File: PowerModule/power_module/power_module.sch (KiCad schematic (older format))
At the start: 1 part

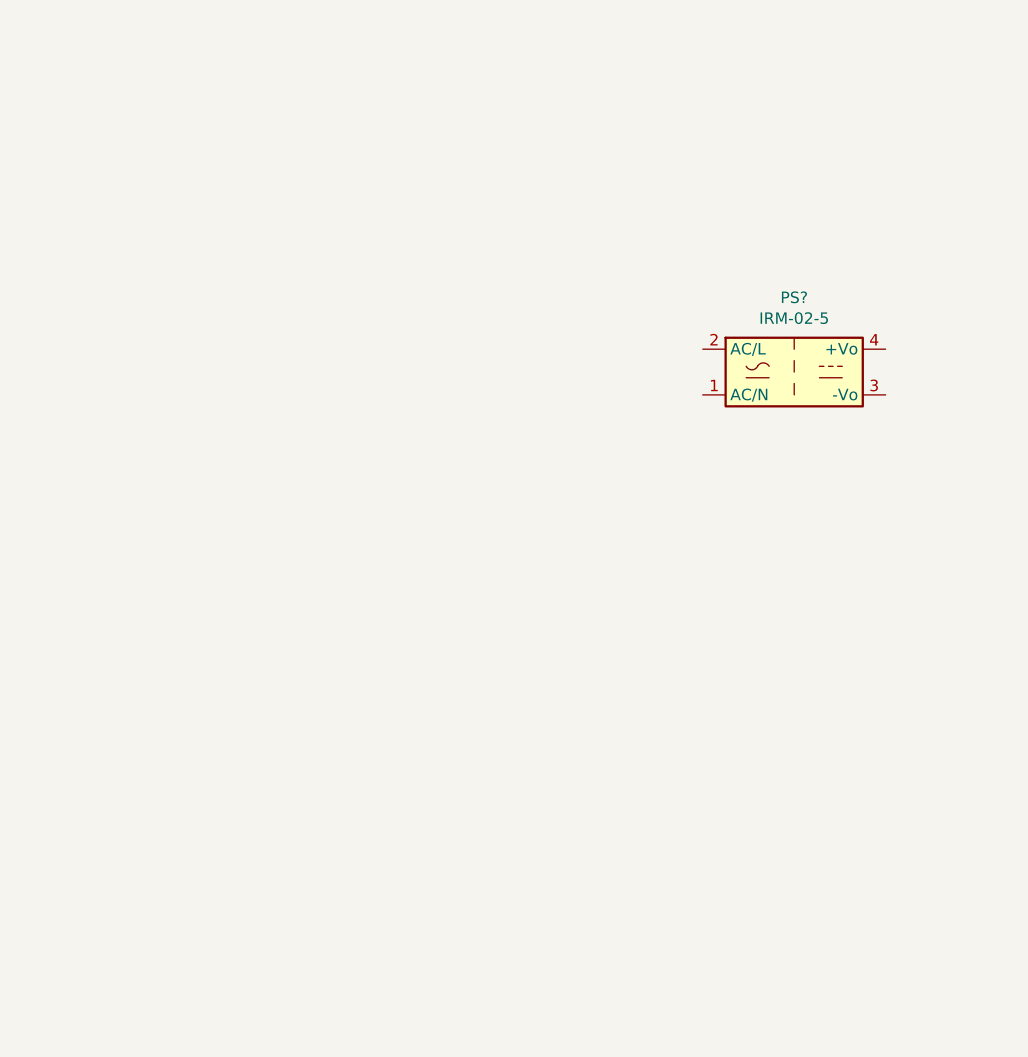
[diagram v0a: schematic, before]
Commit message: Работа над схемой. Добавлены файлы документации на реле
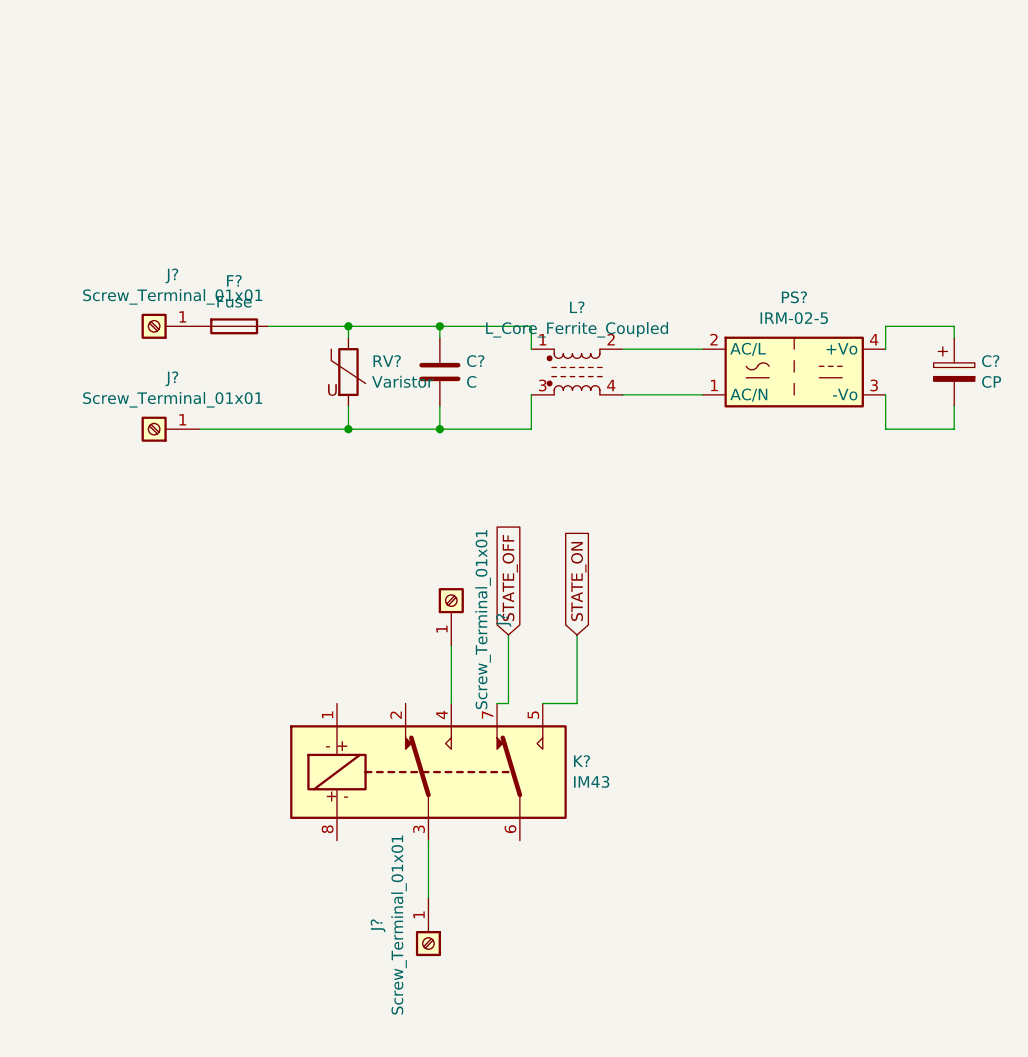
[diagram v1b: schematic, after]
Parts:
- added C?: C, symbol Device:C
- added C?: CP, symbol Device:CP
- added F?: Fuse, symbol Device:Fuse
- added J? (x4): Screw_Terminal_01x01, symbol Connector:Screw_Terminal_01x01
- added K?: IM43, symbol Relay:IM43
- added L?: L_Core_Ferrite_Coupled, symbol Device:L_Core_Ferrite_Coupled
- added RV?: Varistor, symbol Device:Varistor
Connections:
- net at PS?.1 (AC/N): now also L?.4
- net at PS?.2 (AC/L): now also L?.2
- net at PS?.3 (-Vo): now also C?.2
- net at PS?.4 (+Vo): now also C?.1
- new net: C?.1, F?.1, L?.1, RV?.1
- new net: C?.2, J?.1 (Pin_1), L?.3, RV?.2
- new net: F?.2, J?.1 (Pin_1)
- new net: J?.1 (Pin_1), K?.3
- new net: J?.1 (Pin_1), K?.4
- new net STATE_OFF: K?.7
- new net STATE_ON: K?.5
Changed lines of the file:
@@
 	1    0    0    -1
 $EndComp
+$Comp
+L Device:L_Core_Ferrite_Coupled L?
+U 1 1 5FD75833
+P 3000 2750
+F 0 "L?" H 3000 3031 50  0000 C CNN
+F 1 "L_Core_Ferrite_Coupled" H 3000 2940 50  0000 C CNN
+F 2 "" H 3000 2750 50  0001 C CNN
+F 3 "~" H 3000 2750 50  0001 C CNN
+	1    3000 2750
+	1    0    0    -1
+$EndComp
+$Comp
+L Device:C C?
+U 1 1 5FD7B6BD
+P 2400 2750
+F 0 "C?" H 2515 2796 50  0000 L CNN
+F 1 "C" H 2515 2705 50  0000 L CNN
+F 2 "" H 2438 2600 50  0001 C CNN
+F 3 "~" H 2400 2750 50  0001 C CNN
+	1    2400 2750
+	1    0    0    -1
+$EndComp
+$Comp
+L Device:Varistor RV?
+U 1 1 5FD7BDB9
+P 2000 2750
+F 0 "RV?" H 2103 2796 50  0000 L CNN
+F 1 "Varistor" H 2103 2705 50  0000 L CNN
+F 2 "" V 1930 2750 50  0001 C CNN
+F 3 "~" H 2000 2750 50  0001 C CNN
+	1    2000 2750
+	1    0    0    -1
+$EndComp
+$Comp
+L Device:Fuse F?
+U 1 1 5FD7C7CC
+P 1500 2550
+F 0 "F?" V 1303 2550 50  0000 C CNN
+F 1 "Fuse" V 1394 2550 50  0000 C CNN
+F 2 "" V 1430 2550 50  0001 C CNN
+F 3 "~" H 1500 2550 50  0001 C CNN
+	1    1500 2550
+	0    1    1    0
+$EndComp
+Wire Wire Line
+	1650 2550 2000 2550
+Wire Wire Line
+	2400 2550 2400 2600
+Wire Wire Line
+	2000 2600 2000 2550
+Connection ~ 2000 2550
+Wire Wire Line
+	2000 2550 2400 2550
+Wire Wire Line
+	2800 2650 2800 2550
+Wire Wire Line
+	2800 2550 2400 2550
+Connection ~ 2400 2550
+Wire Wire Line
+	2800 2850 2800 3000
+Wire Wire Line
+	2800 3000 2400 3000
+Wire Wire Line
+	2400 3000 2400 2900
+Wire Wire Line
+	2400 3000 2000 3000
+Wire Wire Line
+	2000 3000 2000 2900
+Connection ~ 2400 3000
+$Comp
+L Connector:Screw_Terminal_01x01 J?
+U 1 1 5FD7E4B3
+P 1150 2550
+F 0 "J?" H 1068 2325 50  0000 C CNN
+F 1 "Screw_Terminal_01x01" H 1068 2416 50  0000 C CNN
+F 2 "" H 1150 2550 50  0001 C CNN
+F 3 "~" H 1150 2550 50  0001 C CNN
+	1    1150 2550
+	-1   0    0    1
+$EndComp
+$Comp
+L Connector:Screw_Terminal_01x01 J?
+U 1 1 5FD7F068
+P 1150 3000
+F 0 "J?" H 1068 2775 50  0000 C CNN
+F 1 "Screw_Terminal_01x01" H 1068 2866 50  0000 C CNN
+F 2 "" H 1150 3000 50  0001 C CNN
+F 3 "~" H 1150 3000 50  0001 C CNN
+	1    1150 3000
+	-1   0    0    1
+$EndComp
+Wire Wire Line
+	2000 3000 1350 3000
+Connection ~ 2000 3000
+Wire Wire Line
+	3550 2650 3200 2650
+Wire Wire Line
+	3550 2850 3200 2850
+$Comp
+L Device:CP C?
+U 1 1 5FD807F1
+P 4650 2750
+F 0 "C?" H 4768 2796 50  0000 L CNN
+F 1 "CP" H 4768 2705 50  0000 L CNN
+F 2 "" H 4688 2600 50  0001 C CNN
+F 3 "~" H 4650 2750 50  0001 C CNN
+	1    4650 2750
+	1    0    0    -1
+$EndComp
+Wire Wire Line
+	4350 2650 4350 2550
+Wire Wire Line
+	4350 2550 4650 2550
+Wire Wire Line
+	4650 2550 4650 2600
+Wire Wire Line
+	4350 2850 4350 3000
+Wire Wire Line
+	4350 3000 4650 3000
+Wire Wire Line
+	4650 3000 4650 2900
+$Comp
+L Relay:IM43 K?
+U 1 1 5FD824A3
+P 2350 4500
+F 0 "K?" H 2980 4546 50  0000 L CNN
+F 1 "IM43" H 2980 4455 50  0000 L CNN
+F 2 "" H 2350 4500 50  0001 C CNN
+F 3 "http://www.te.com/commerce/DocumentDelivery/DDEController?Action=srchrtrv&DocNm=108-98001&DocType=SS&DocLang=EN" H 2350 4500 50  0001 C CNN
+	1    2350 4500
+	1    0    0    -1
+$EndComp
+$Comp
+L Connector:Screw_Terminal_01x01 J?
+U 1 1 5FD84611
+P 2450 3750
+F 0 "J?" H 2368 3525 50  0000 C CNN
+F 1 "Screw_Terminal_01x01" H 2368 3616 50  0000 C CNN
+F 2 "" H 2450 3750 50  0001 C CNN
+F 3 "~" H 2450 3750 50  0001 C CNN
+	1    2450 3750
+	0    -1   -1   0
+$EndComp
+$Comp
+L Connector:Screw_Terminal_01x01 J?
+U 1 1 5FD84B7D
+P 2350 5250
+F 0 "J?" H 2268 5025 50  0000 C CNN
+F 1 "Screw_Terminal_01x01" H 2268 5116 50  0000 C CNN
+F 2 "" H 2350 5250 50  0001 C CNN
+F 3 "~" H 2350 5250 50  0001 C CNN
+	1    2350 5250
+	0    1    1    0
+$EndComp
+Wire Wire Line
+	2350 5050 2350 4800
+Wire Wire Line
+	2450 4200 2450 3950
+Text GLabel 2700 3900 1    50   Input ~ 0
+STATE_OFF
+Text GLabel 3000 3900 1    50   Input ~ 0
+STATE_ON
+Wire Wire Line
+	2650 4200 2700 4200
+Wire Wire Line
+	2700 4200 2700 3900
+Wire Wire Line
+	2850 4200 3000 4200
+Wire Wire Line
+	3000 4200 3000 3900
 $EndSCHEMATC

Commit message: Update
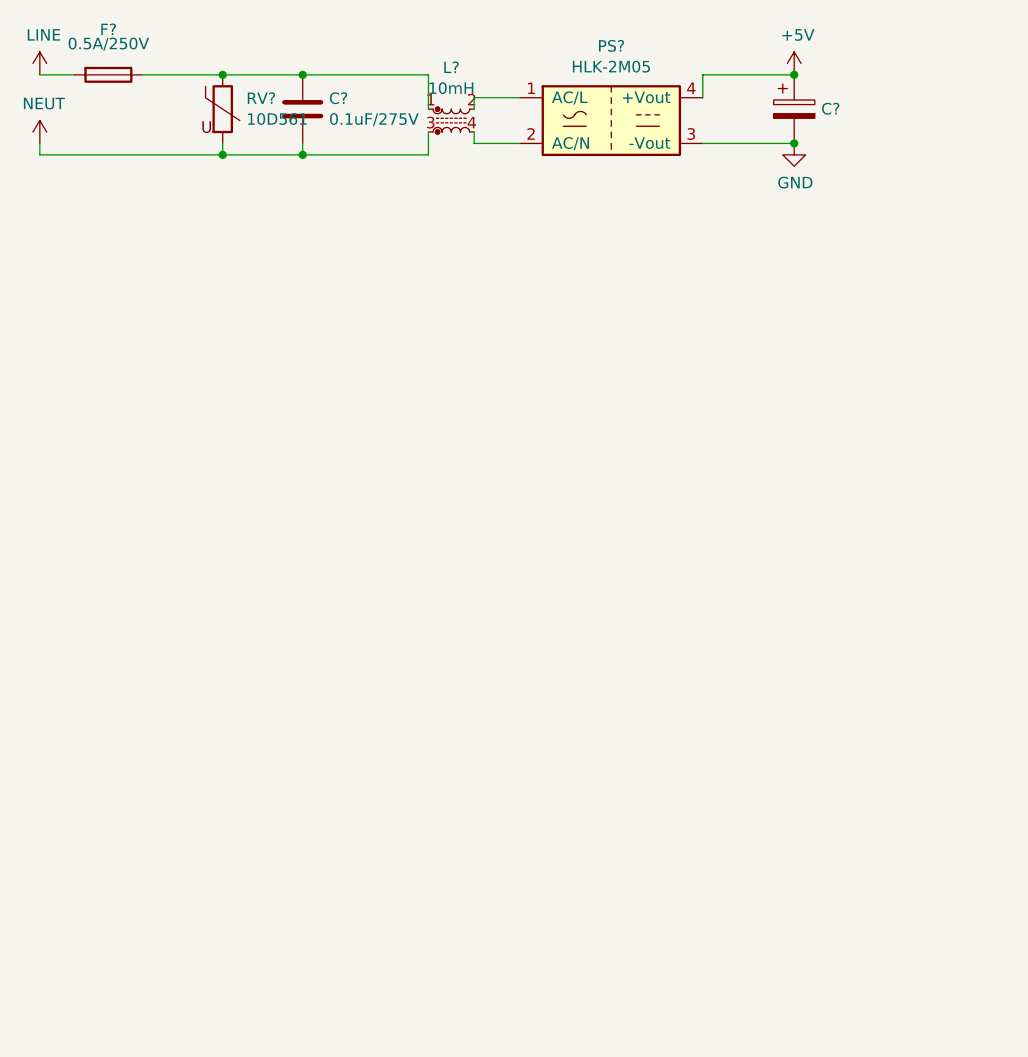
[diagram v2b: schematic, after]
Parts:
- removed C?: C, symbol Device:C
- removed C?: CP, symbol Device:CP
- removed F?: Fuse, symbol Device:Fuse
- removed J? (x4): Screw_Terminal_01x01, symbol Connector:Screw_Terminal_01x01
- removed K?: IM43, symbol Relay:IM43
- removed L?: L_Core_Ferrite_Coupled, symbol Device:L_Core_Ferrite_Coupled
- removed PS?: IRM-02-5, Converter_ACDC:Converter_ACDC_MeanWell_IRM-02-xx_THT, symbol Converter_ACDC:IRM-02-5
- removed RV?: Varistor, symbol Device:Varistor
- added C?: 0.1uF/275V, symbol Device:C
- added C?: CP, symbol Device:CP
- added F?: 0.5A/250V, symbol Device:Fuse
- added L?: 10mH, symbol Device:L_Core_Ferrite_Coupled_Small
- added PS?: HLK-2M05, symbol HLK-2M05:HLK-2M05
- added RV?: 10D561, symbol Device:Varistor
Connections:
- new net: L?.2, PS?.1 (AC/L)
- new net: L?.4, PS?.2 (AC/N)
- new net: C?.1, F?.1, L?.1, RV?.1
- new net +5V: C?.1, PS?.4 (+Vout)
- new net GND: C?.2, PS?.3 (-Vout)
- new net LINE: F?.2
- new net NEUT: C?.2, L?.3, RV?.2
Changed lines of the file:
@@
 $EndDescr
 $Comp
-L Converter_ACDC:IRM-02-5 PS?
-U 1 1 5F7C2639
-P 3950 2750
-F 0 "PS?" H 3950 3075 50  0000 C CNN
-F 1 "IRM-02-5" H 3950 2984 50  0000 C CNN
-F 2 "Converter_ACDC:Converter_ACDC_MeanWell_IRM-02-xx_THT" H 3950 2450 50  0001 C CNN
-F 3 "https://www.meanwell.com/Upload/PDF/IRM-02/IRM-02-SPEC.PDF" H 4350 2400 50  0001 C CNN
-	1    3950 2750
+L HLK-2M05:HLK-2M05 PS?
+U 1 1 5EC3E9C7
+P 3150 1650
+F 0 "PS?" H 3150 1975 50  0000 C CNN
+F 1 "HLK-2M05" H 3150 1884 50  0000 C CNN
+F 2 "" H 3150 1650 50  0001 C CNN
+F 3 "" H 3150 1650 50  0001 C CNN
+	1    3150 1650
 	1    0    0    -1
 $EndComp
 $Comp
-L Device:L_Core_Ferrite_Coupled L?
-U 1 1 5FD75833
-P 3000 2750
-F 0 "L?" H 3000 3031 50  0000 C CNN
-F 1 "L_Core_Ferrite_Coupled" H 3000 2940 50  0000 C CNN
-F 2 "" H 3000 2750 50  0001 C CNN
-F 3 "~" H 3000 2750 50  0001 C CNN
-	1    3000 2750
+L Device:L_Core_Ferrite_Coupled_Small L?
+U 1 1 5EC4009B
+P 2450 1650
+F 0 "L?" H 2450 1881 50  0000 C CNN
+F 1 "10mH" H 2450 1790 50  0000 C CNN
+F 2 "" H 2450 1650 50  0001 C CNN
+F 3 "http://www.kosmodrom.com.ua/el.php?name=DLF-103U-1A" H 2450 1650 50  0001 C CNN
+	1    2450 1650
 	1    0    0    -1
 $EndComp
 $Comp
 L Device:C C?
-U 1 1 5FD7B6BD
-P 2400 2750
-F 0 "C?" H 2515 2796 50  0000 L CNN
-F 1 "C" H 2515 2705 50  0000 L CNN
-F 2 "" H 2438 2600 50  0001 C CNN
-F 3 "~" H 2400 2750 50  0001 C CNN
-	1    2400 2750
+U 1 1 5EC41904
+P 1800 1600
+F 0 "C?" H 1915 1646 50  0000 L CNN
+F 1 "0.1uF/275V" H 1915 1555 50  0000 L CNN
+F 2 "" H 1838 1450 50  0001 C CNN
+F 3 "~" H 1800 1600 50  0001 C CNN
+	1    1800 1600
 	1    0    0    -1
 $EndComp
 $Comp
 L Device:Varistor RV?
-U 1 1 5FD7BDB9
-P 2000 2750
-F 0 "RV?" H 2103 2796 50  0000 L CNN
-F 1 "Varistor" H 2103 2705 50  0000 L CNN
-F 2 "" V 1930 2750 50  0001 C CNN
-F 3 "~" H 2000 2750 50  0001 C CNN
-	1    2000 2750
+U 1 1 5EC42913
+P 1450 1600
+F 0 "RV?" H 1553 1646 50  0000 L CNN
+F 1 "10D561" H 1553 1555 50  0000 L CNN
+F 2 "" V 1380 1600 50  0001 C CNN
+F 3 "~" H 1450 1600 50  0001 C CNN
+	1    1450 1600
 	1    0    0    -1
 $EndComp
 $Comp
 L Device:Fuse F?
-U 1 1 5FD7C7CC
-P 1500 2550
-F 0 "F?" V 1303 2550 50  0000 C CNN
-F 1 "Fuse" V 1394 2550 50  0000 C CNN
-F 2 "" V 1430 2550 50  0001 C CNN
-F 3 "~" H 1500 2550 50  0001 C CNN
-	1    1500 2550
+U 1 1 5EC433D5
+P 950 1450
+F 0 "F?" V 753 1450 50  0000 C CNN
+F 1 "0.5A/250V" V 844 1450 50  0000 C BNN
+F 2 "" V 880 1450 50  0001 C CNN
+F 3 "http://www.kosmodrom.com.ua/prodlist.php?name=fuseaxiallead" H 950 1450 50  0001 C CNN
+	1    950  1450
 	0    1    1    0
 $EndComp
-Wire Wire Line
-	1650 2550 2000 2550
-Wire Wire Line
-	2400 2550 2400 2600
-Wire Wire Line
-	2000 2600 2000 2550
-Connection ~ 2000 2550
-Wire Wire Line
-	2000 2550 2400 2550
-Wire Wire Line
-	2800 2650 2800 2550
-Wire Wire Line
-	2800 2550 2400 2550
-Connection ~ 2400 2550
-Wire Wire Line
-	2800 2850 2800 3000
-Wire Wire Line
-	2800 3000 2400 3000
-Wire Wire Line
-	2400 3000 2400 2900
-Wire Wire Line
-	2400 3000 2000 3000
-Wire Wire Line
-	2000 3000 2000 2900
-Connection ~ 2400 3000
-$Comp
-L Connector:Screw_Terminal_01x01 J?
-U 1 1 5FD7E4B3
-P 1150 2550
-F 0 "J?" H 1068 2325 50  0000 C CNN
-F 1 "Screw_Terminal_01x01" H 1068 2416 50  0000 C CNN
-F 2 "" H 1150 2550 50  0001 C CNN
-F 3 "~" H 1150 2550 50  0001 C CNN
-	1    1150 2550
-	-1   0    0    1
-$EndComp
-$Comp
-L Connector:Screw_Terminal_01x01 J?
-U 1 1 5FD7F068
-P 1150 3000
-F 0 "J?" H 1068 2775 50  0000 C CNN
-F 1 "Screw_Terminal_01x01" H 1068 2866 50  0000 C CNN
-F 2 "" H 1150 3000 50  0001 C CNN
-F 3 "~" H 1150 3000 50  0001 C CNN
-	1    1150 3000
-	-1   0    0    1
-$EndComp
-Wire Wire Line
-	2000 3000 1350 3000
-Connection ~ 2000 3000
-Wire Wire Line
-	3550 2650 3200 2650
-Wire Wire Line
-	3550 2850 3200 2850
 $Comp
 L Device:CP C?
-U 1 1 5FD807F1
-P 4650 2750
-F 0 "C?" H 4768 2796 50  0000 L CNN
-F 1 "CP" H 4768 2705 50  0000 L CNN
-F 2 "" H 4688 2600 50  0001 C CNN
-F 3 "~" H 4650 2750 50  0001 C CNN
-	1    4650 2750
+U 1 1 5EC44005
+P 3950 1600
+F 0 "C?" H 4068 1600 50  0000 L CNN
+F 1 "CP" H 4068 1555 50  0001 L CNN
+F 2 "" H 3988 1450 50  0001 C CNN
+F 3 "~" H 3950 1600 50  0001 C CNN
+	1    3950 1600
 	1    0    0    -1
 $EndComp
 Wire Wire Line
-	4350 2650 4350 2550
+	2550 1600 2550 1550
 Wire Wire Line
-	4350 2550 4650 2550
+	2550 1550 2750 1550
 Wire Wire Line
-	4650 2550 4650 2600
+	2750 1750 2550 1750
 Wire Wire Line
-	4350 2850 4350 3000
+	2550 1750 2550 1700
 Wire Wire Line
-	4350 3000 4650 3000
+	2350 1600 2350 1450
 Wire Wire Line
-	4650 3000 4650 2900
+	2350 1450 1800 1450
+Wire Wire Line
+	2350 1700 2350 1800
+Wire Wire Line
+	2350 1800 1800 1800
+Wire Wire Line
+	1800 1800 1800 1750
+Wire Wire Line
+	1800 1800 1450 1800
+Wire Wire Line
+	1450 1800 1450 1750
+Connection ~ 1800 1800
+Wire Wire Line
+	1800 1450 1450 1450
+Connection ~ 1800 1450
+Wire Wire Line
+	1100 1450 1450 1450
+Connection ~ 1450 1450
+Wire Wire Line
+	3950 1750 3550 1750
+Wire Wire Line
+	3550 1550 3550 1450
+Wire Wire Line
+	3550 1450 3950 1450
 $Comp
-L Relay:IM43 K?
-U 1 1 5FD824A3
-P 2350 4500
-F 0 "K?" H 2980 4546 50  0000 L CNN
-F 1 "IM43" H 2980 4455 50  0000 L CNN
-F 2 "" H 2350 4500 50  0001 C CNN
-F 3 "http://www.te.com/commerce/DocumentDelivery/DDEController?Action=srchrtrv&DocNm=108-98001&DocType=SS&DocLang=EN" H 2350 4500 50  0001 C CNN
-	1    2350 4500
+L power:GND #PWR?
+U 1 1 5EC47B87
+P 3950 1750
+F 0 "#PWR?" H 3950 1500 50  0001 C CNN
+F 1 "GND" H 3955 1577 50  0000 C CNN
+F 2 "" H 3950 1750 50  0001 C CNN
+F 3 "" H 3950 1750 50  0001 C CNN
+	1    3950 1750
+	1    0    0    -1
+$EndComp
+Connection ~ 3950 1750
+$Comp
+L power:+5V #PWR?
+U 1 1 5EC4831F
+P 3950 1450
+F 0 "#PWR?" H 3950 1300 50  0001 C CNN
+F 1 "+5V" H 3965 1623 50  0000 C CNN
+F 2 "" H 3950 1450 50  0001 C CNN
+F 3 "" H 3950 1450 50  0001 C CNN
+	1    3950 1450
+	1    0    0    -1
+$EndComp
+Connection ~ 3950 1450
+$Comp
+L power:LINE #PWR?
+U 1 1 5EC4A041
+P 650 1450
+F 0 "#PWR?" H 650 1300 50  0001 C CNN
+F 1 "LINE" H 667 1623 50  0000 C CNN
+F 2 "" H 650 1450 50  0001 C CNN
+F 3 "" H 650 1450 50  0001 C CNN
+	1    650  1450
 	1    0    0    -1
 $EndComp
 $Comp
-L Connector:Screw_Terminal_01x01 J?
-U 1 1 5FD84611
-P 2450 3750
-F 0 "J?" H 2368 3525 50  0000 C CNN
-F 1 "Screw_Terminal_01x01" H 2368 3616 50  0000 C CNN
-F 2 "" H 2450 3750 50  0001 C CNN
-F 3 "~" H 2450 3750 50  0001 C CNN
-	1    2450 3750
-	0    -1   -1   0
-$EndComp
-$Comp
-L Connector:Screw_Terminal_01x01 J?
-U 1 1 5FD84B7D
-P 2350 5250
-F 0 "J?" H 2268 5025 50  0000 C CNN
-F 1 "Screw_Terminal_01x01" H 2268 5116 50  0000 C CNN
-F 2 "" H 2350 5250 50  0001 C CNN
-F 3 "~" H 2350 5250 50  0001 C CNN
-	1    2350 5250
-	0    1    1    0
+L power:NEUT #PWR?
+U 1 1 5EC4AACC
+P 650 1750
+F 0 "#PWR?" H 650 1600 50  0001 C CNN
+F 1 "NEUT" H 667 1923 50  0000 C CNN
+F 2 "" H 650 1750 50  0001 C CNN
+F 3 "" H 650 1750 50  0001 C CNN
+	1    650  1750
+	1    0    0    -1
 $EndComp
 Wire Wire Line
-	2350 5050 2350 4800
+	800  1450 650  1450
 Wire Wire Line
-	2450 4200 2450 3950
-Text GLabel 2700 3900 1    50   Input ~ 0
-STATE_OFF
-Text GLabel 3000 3900 1    50   Input ~ 0
-STATE_ON
+	1450 1800 650  1800
 Wire Wire Line
-	2650 4200 2700 4200
-Wire Wire Line
-	2700 4200 2700 3900
-Wire Wire Line
-	2850 4200 3000 4200
-Wire Wire Line
-	3000 4200 3000 3900
+	650  1800 650  1750
+Connection ~ 1450 1800
 $EndSCHEMATC
